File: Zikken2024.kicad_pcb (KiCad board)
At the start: 2 copper layers, 41 parts, among them J2 sensor1, J5 sensor2, J6 sensor3, J8 sensor4, Q1 2SC1815, U3 SM420561N

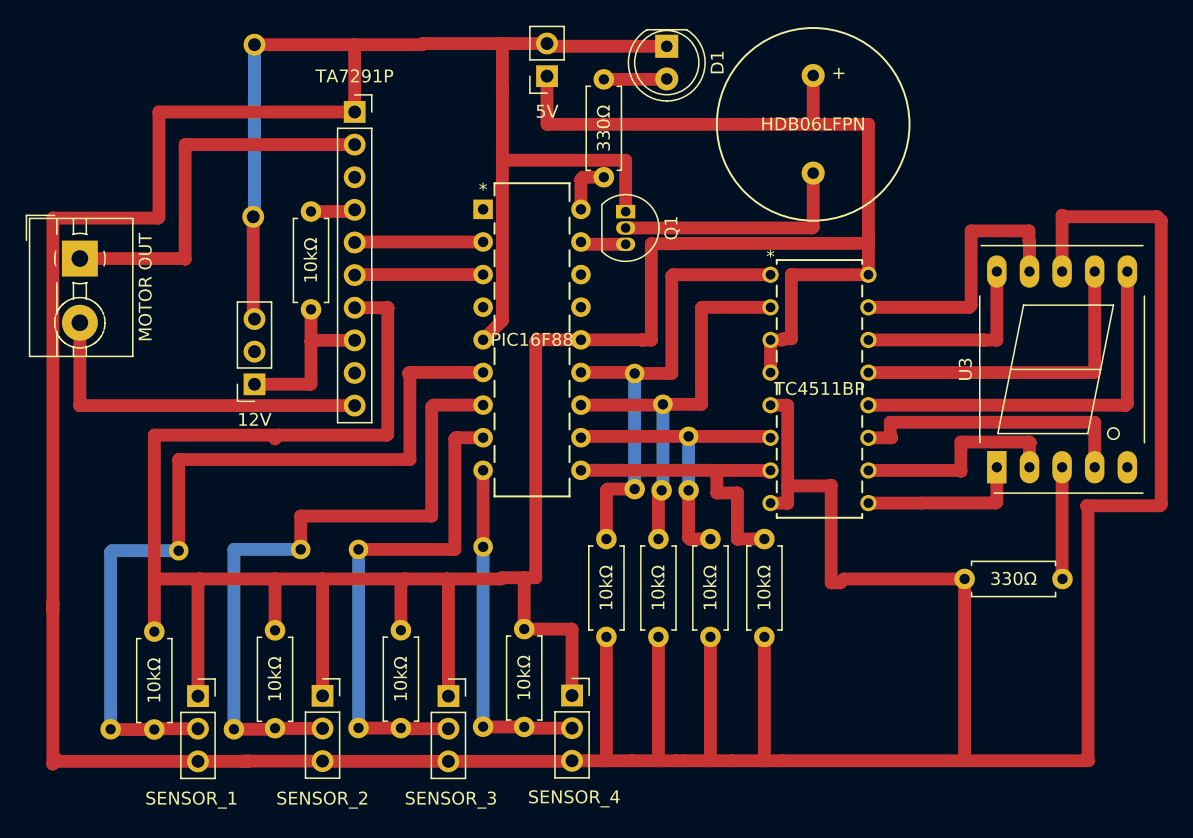
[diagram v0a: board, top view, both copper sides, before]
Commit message: update track
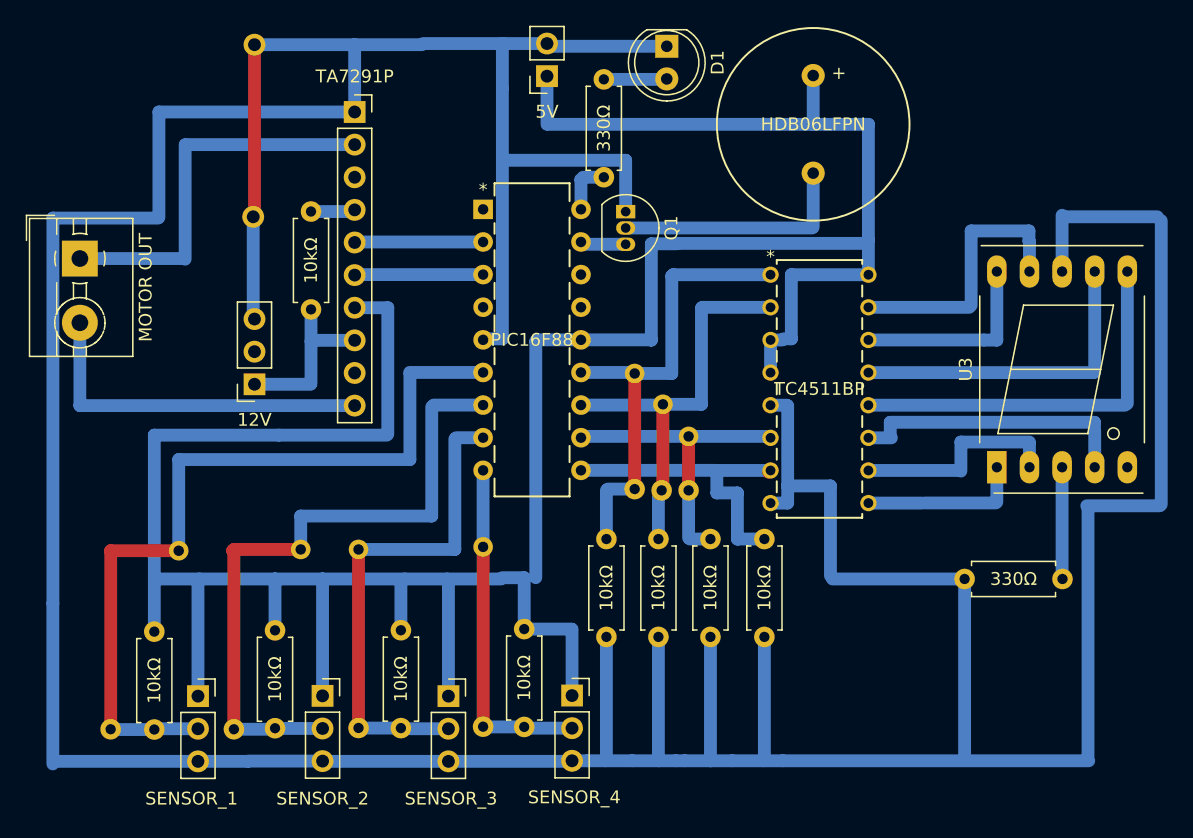
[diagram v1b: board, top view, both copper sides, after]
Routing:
- net GND: track 397.4 -> 393.9 mm
- net 5V: track 236.6 -> 233.6 mm
